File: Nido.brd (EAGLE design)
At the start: 26.3 x 16 mm, 10 parts, among them K1 HE3621, T1 BC337, U1 BME280

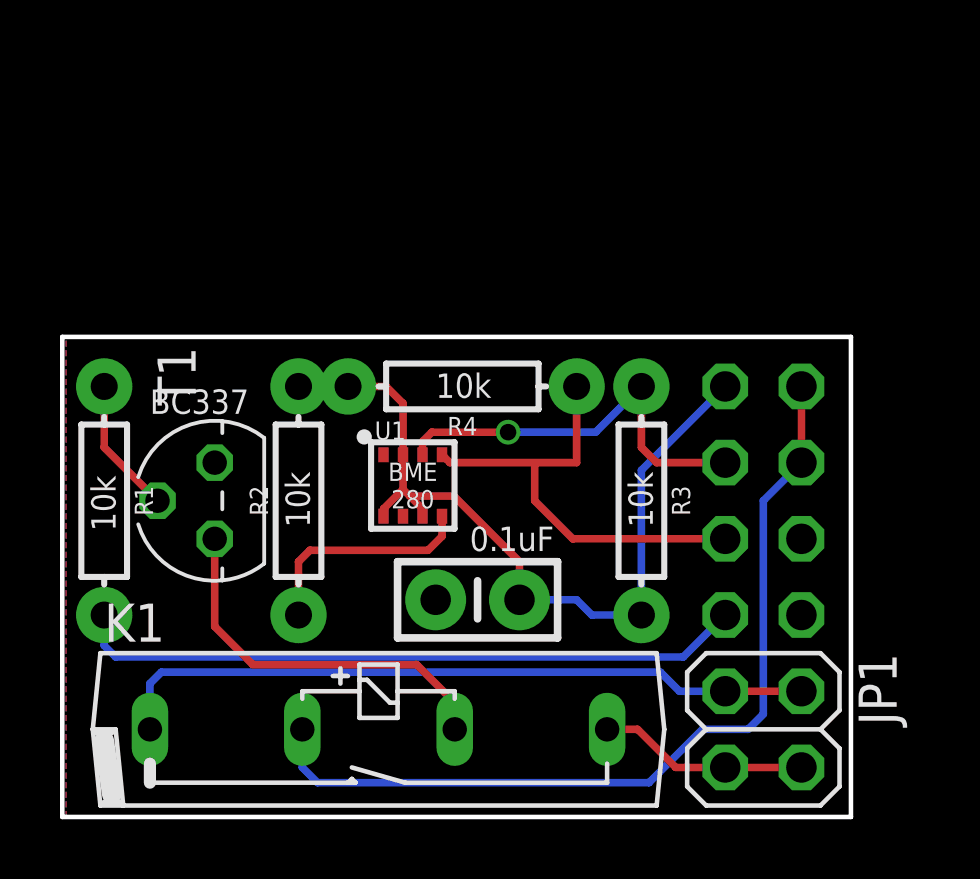
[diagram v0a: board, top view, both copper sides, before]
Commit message: Updated Nido PCB v2 files
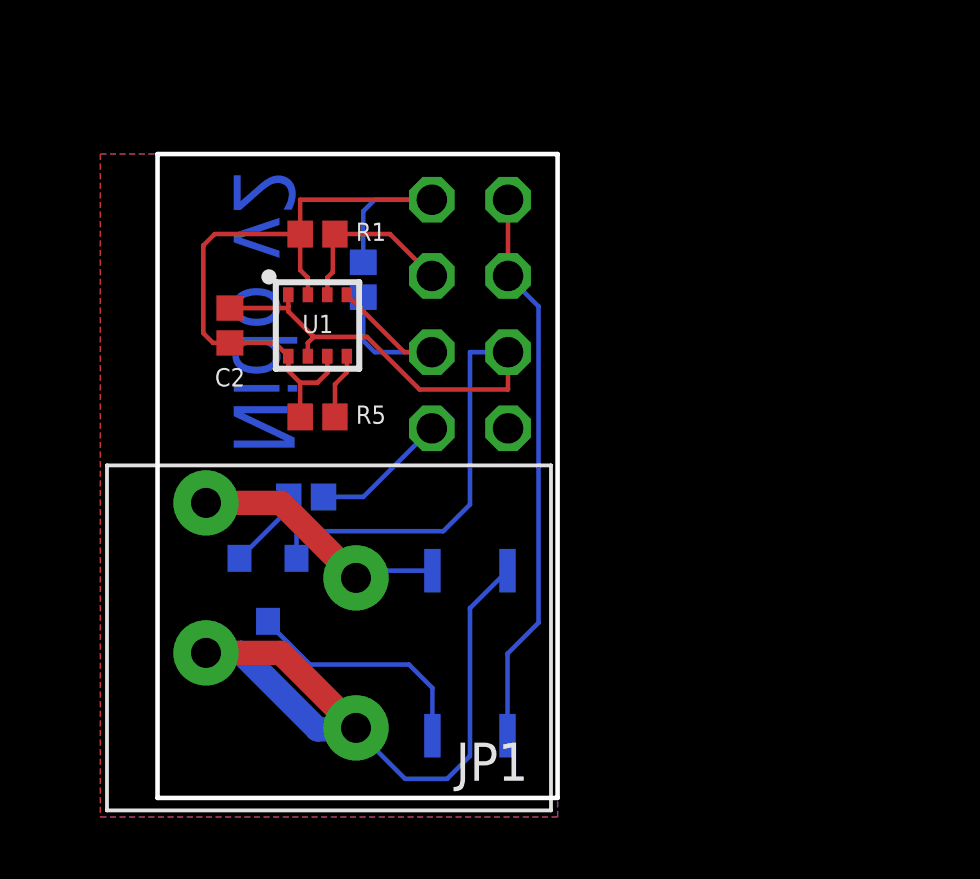
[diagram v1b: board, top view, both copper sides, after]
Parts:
- removed C1: 0.1uF, SparkFun-Capacitors:CAP-PTH-SMALL-KIT
- removed K1: HE3621, relay:HE3621
- removed R4: 10k, SparkFun-Resistors:AXIAL-0.3
- removed T1: BC337, transistor:TO92
- added C2: 0.1uF, SparkFun-Capacitors:0402
- added Q1: 500mA/300V, SparkFun-DiscreteSemi:SOT23-3
- added R5: 10k, SparkFun-Resistors:0402
- added U2: CPC1017NSOP4, nido:CPC1017N
- JP1: value (none) -> 1986712-2TH; device pinhead:2X02 -> nido:1986712-2
- R1, R2, R3: device SparkFun-Resistors:AXIAL-0.3 -> SparkFun-Resistors:0402
- moved JP1 14.8 mm to (8.76, 5.97), turned to 90 degrees
- moved JP2 11.6 mm to (13.5, 16.8)
- moved R1 11.4 mm to (8.38, 19.4), turned to 180 degrees
- moved R3 11.2 mm to (8.00, 10.7), flipped to the bottom, turned to 180 degrees
- moved R2 7.68 mm to (9.91, 17.9), flipped to the bottom
- moved U1 6.21 mm to (8.38, 16.4)
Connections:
- net 3V3: now also C2.1, R1.2, R2.2, R5.2; no longer C1.1, R2.P$2, R3.P$2, R4.P$2
- net 5V: now also U2.1; no longer K1.2
- net GND: now also C2.2, Q1.2; no longer C1.2, T1.1
- net GPIO_4: now also R3.2; no longer R1.P$2
- net HEATER1: now also JP1.P$1, JP1.P$2, U2.4; no longer JP1.1, JP1.2, K1.1
- net HEATER2: now also JP1.P$3, JP1.P$4, U2.3; no longer JP1.3, JP1.4, K1.4
- net N$1: now also R5.1; no longer R2.P$1
- net N$5: now also Q1.3, U2.2; no longer K1.3, T1.3
- net N$6: now also Q1.1, R3.1; no longer R1.P$1, T1.2
- net SCL: now also R2.1; no longer R4.P$1
- net SDA: now also R1.1; no longer R3.P$1
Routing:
- net GND: track 0.00 -> 26.3 mm
- net GPIO_4: track 22.5 -> 4.56 mm
- net 5V: track 29.2 -> 18.7 mm
- net SCL: track 15.3 -> 7.52 mm
- net SDA: track 13.5 -> 5.94 mm, vias 1 -> 0
- net N$1: track 7.58 -> 2.19 mm
- net N$5: track 12.9 -> 8.01 mm
- net 3V3: track 27.8 -> 25.1 mm
- net N$6: track 4.55 -> 2.73 mm
- net HEATER2: track 7.00 -> 8.68 mm
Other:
- board size 26.3 x 16 mm -> 13.3 x 21.5 mm
- board text added: "Nido v2"
- board text removed: "0.1uF"
- board text removed: "10k"
- board text removed: "BC337"
- board text removed: "BME 280"
- board text removed: "Nido v1.0"
- board text removed: "https://github.com/alexmensch/nido"
